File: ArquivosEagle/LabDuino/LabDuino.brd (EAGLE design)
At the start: 97.5 x 68.6 mm, 40 parts, among them IC1 PCF8574P, IC2 PCF8574P

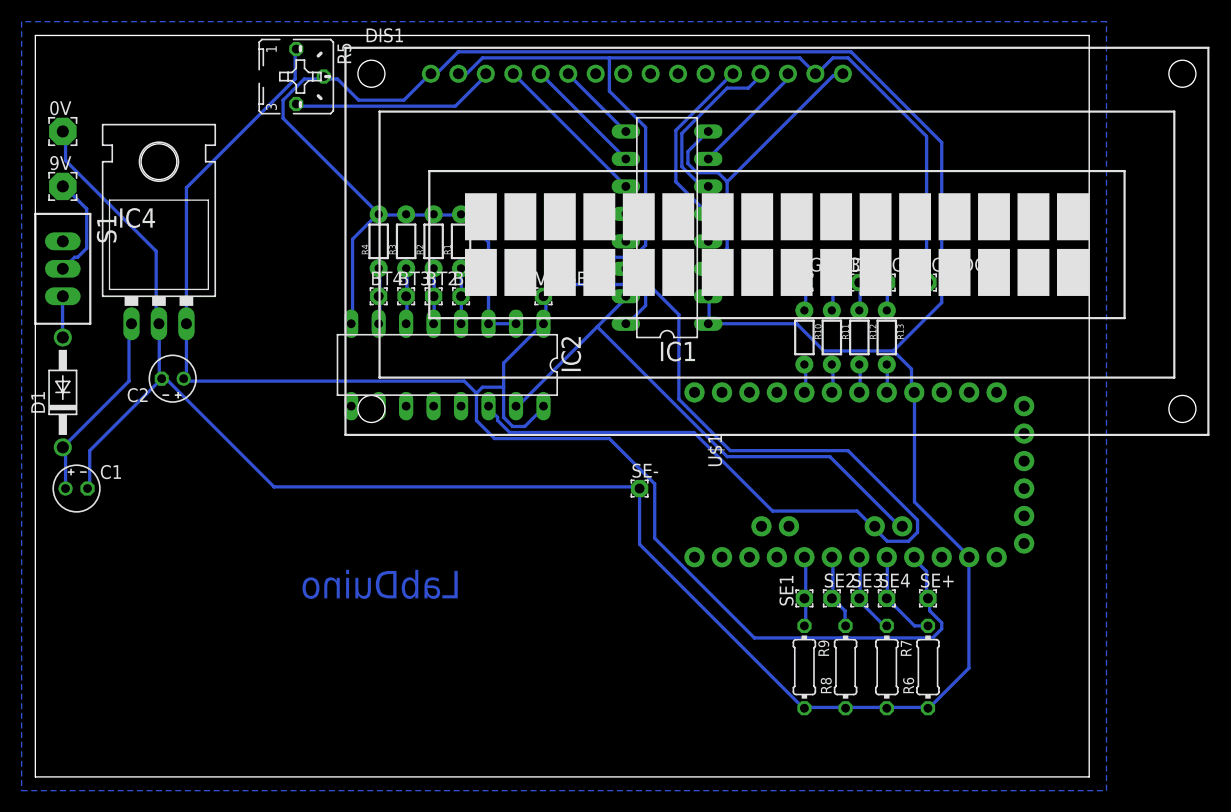
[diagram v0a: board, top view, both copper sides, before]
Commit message: Board Update
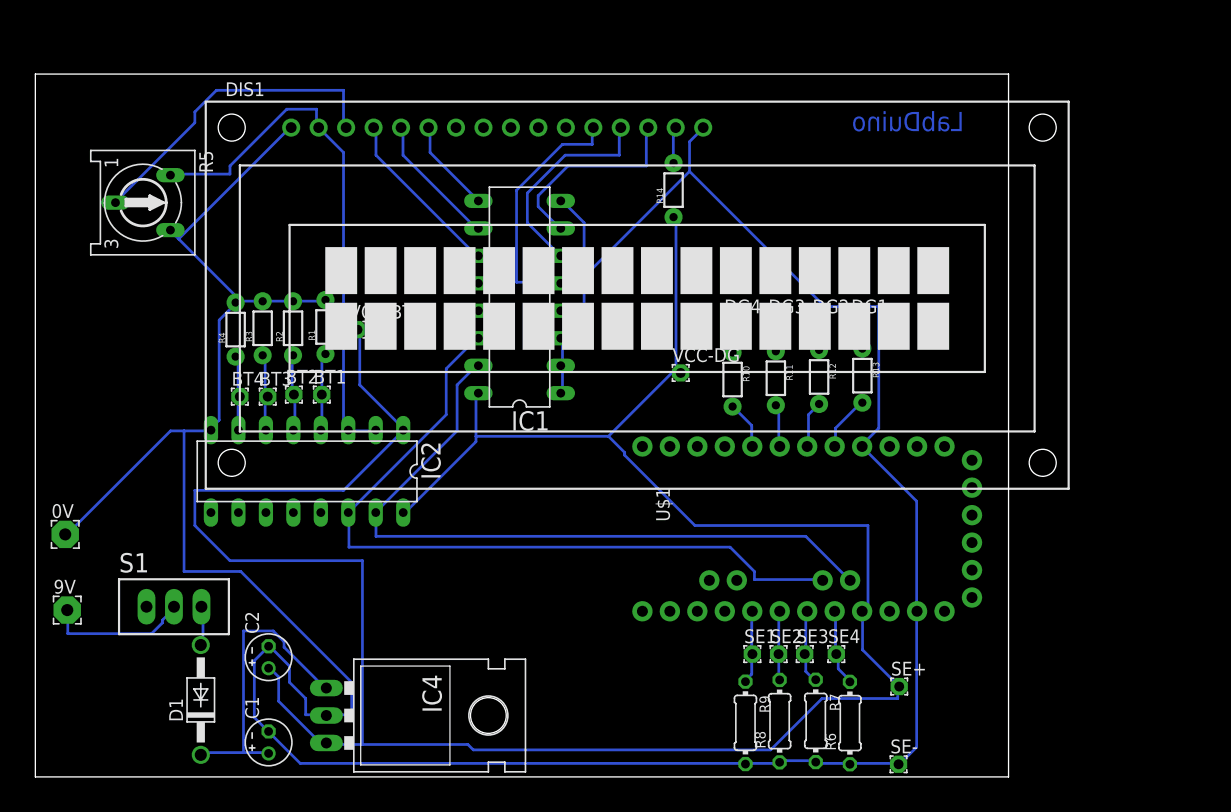
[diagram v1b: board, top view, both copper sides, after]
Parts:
- added R14: (no value), SparkFun-Resistors:1/6W-RES
- R5: device pot:B25P -> pot:RS3
- moved IC4 44.4 mm to (30.7, 5.68), turned to 270 degrees
- moved 9V 39.2 mm to (2.95, 15.4)
- moved 0V 37.3 mm to (2.76, 22.4)
- moved SE- 35.0 mm to (79.8, 1.17)
- moved S1 32.9 mm to (12.8, 15.7), turned to 0 degrees
- moved D1 31.2 mm to (15.3, 7.12)
- moved C1 29.4 mm to (21.6, 3.19), turned to 90 degrees
- moved C2 27.2 mm to (21.6, 11.1), turned to 90 degrees
- moved VCC-DG 24.4 mm to (59.7, 37.4)
- moved R5 18.4 mm to (9.95, 53.1)
- moved VCC-BT 17.5 mm to (29.8, 41.4)
- moved IC2 16.3 mm to (25.1, 28.3)
- moved BT4 15.8 mm to (18.9, 35.2)
- moved BT3 15.8 mm to (21.5, 35.2)
- moved BT2 15.8 mm to (23.9, 35.4)
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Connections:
- new net N$27: DIS1.15, R14.2
- net GND: now also R5.E; no longer R5.S
- net N$14: now also R5.S; no longer R5.E
- net VCC: now also R14.1; no longer DIS1.15
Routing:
- net GND: track 355.6 -> 301.5 mm
- net VCC: track 248.9 -> 268.6 mm
- net SCL: track 87.9 -> 69.9 mm
- net SDA: track 50.5 -> 65.3 mm
- net N$14: track 19.0 -> 29.6 mm
- net N$16: track 18.2 -> 27.8 mm
- net N$10: track 11.1 -> 18.7 mm
- net N$12: track 16.4 -> 23.0 mm
- net N$11: track 15.9 -> 19.7 mm
- net N$3: track 9.67 -> 13.3 mm
- net N$27: track 0.00 -> 3.46 mm
- net N$19: track 2.60 -> 5.14 mm
- net N$2: track 5.16 -> 7.20 mm
- net N$4: track 5.29 -> 7.32 mm
- net 10K: track 5.22 -> 7.09 mm
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- removed copper zone on layer 16, net GND
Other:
- board size 97.5 x 68.6 mm -> 90 x 65 mm
